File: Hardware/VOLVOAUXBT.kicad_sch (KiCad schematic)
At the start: 66 parts, among them J1 10118193-0001LF, J10 Conn_01x02_Pin, J11 Conn_01x02_Pin, J12 Conn_01x05_Pin, J13 Conn_01x05_Pin, J14 Conn_01x05_Pin, J15 Conn_01x02_Pin, J16 Conn_01x02_Pin, J17 Conn_01x01_Pin, J18 Conn_01x02_Pin, J19 Conn_01x01_Pin, J2 10118193-0001LF, J3 F52R-1A7H1-11018, J4 Conn_01x18_Pin, J5 Conn_01x18_Pin, J6 F52R-1A7H1-11018, J7 Conn_01x18_Pin, J8 U_FL-R-SMT_10_, J9 Conn_01x02_Pin, U1 SGM2212-3.3, U2 SGM2212-3.3, U3 TJA1027T_20_118, U4 ESP32-MINI-1, U5 TJA1027T_20_118, U6 SN74AHCT157PWR, U7 CP2102N-Axx-xQFN20

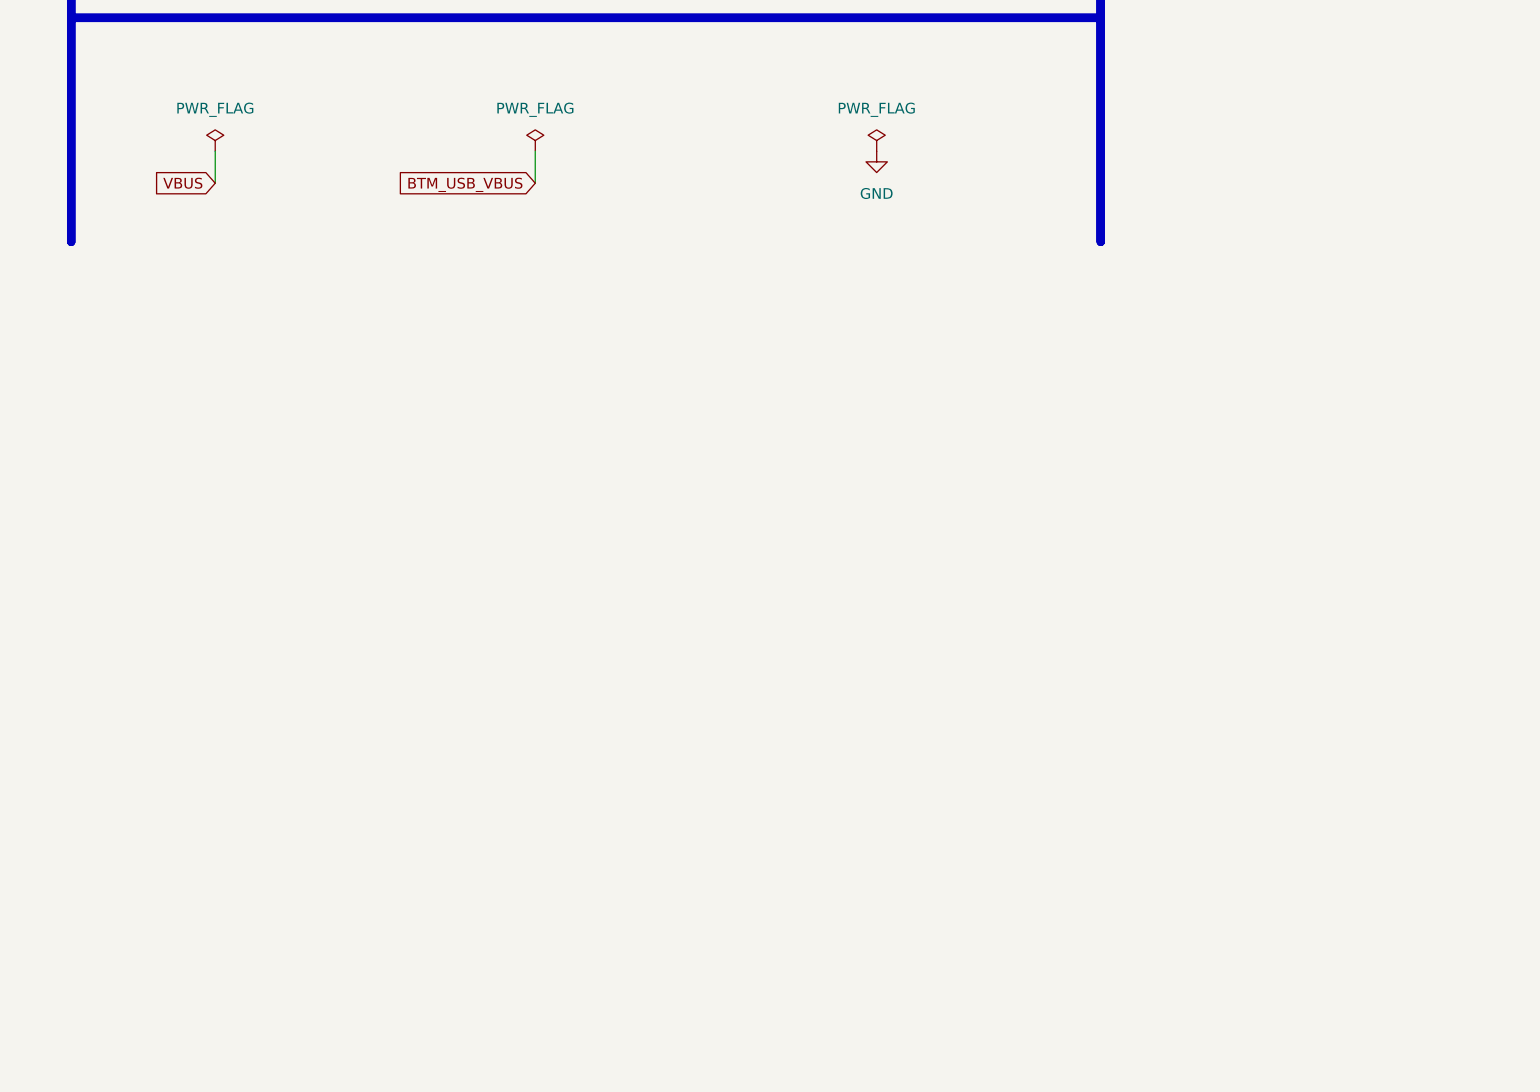
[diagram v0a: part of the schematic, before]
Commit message: Before swap to wroom
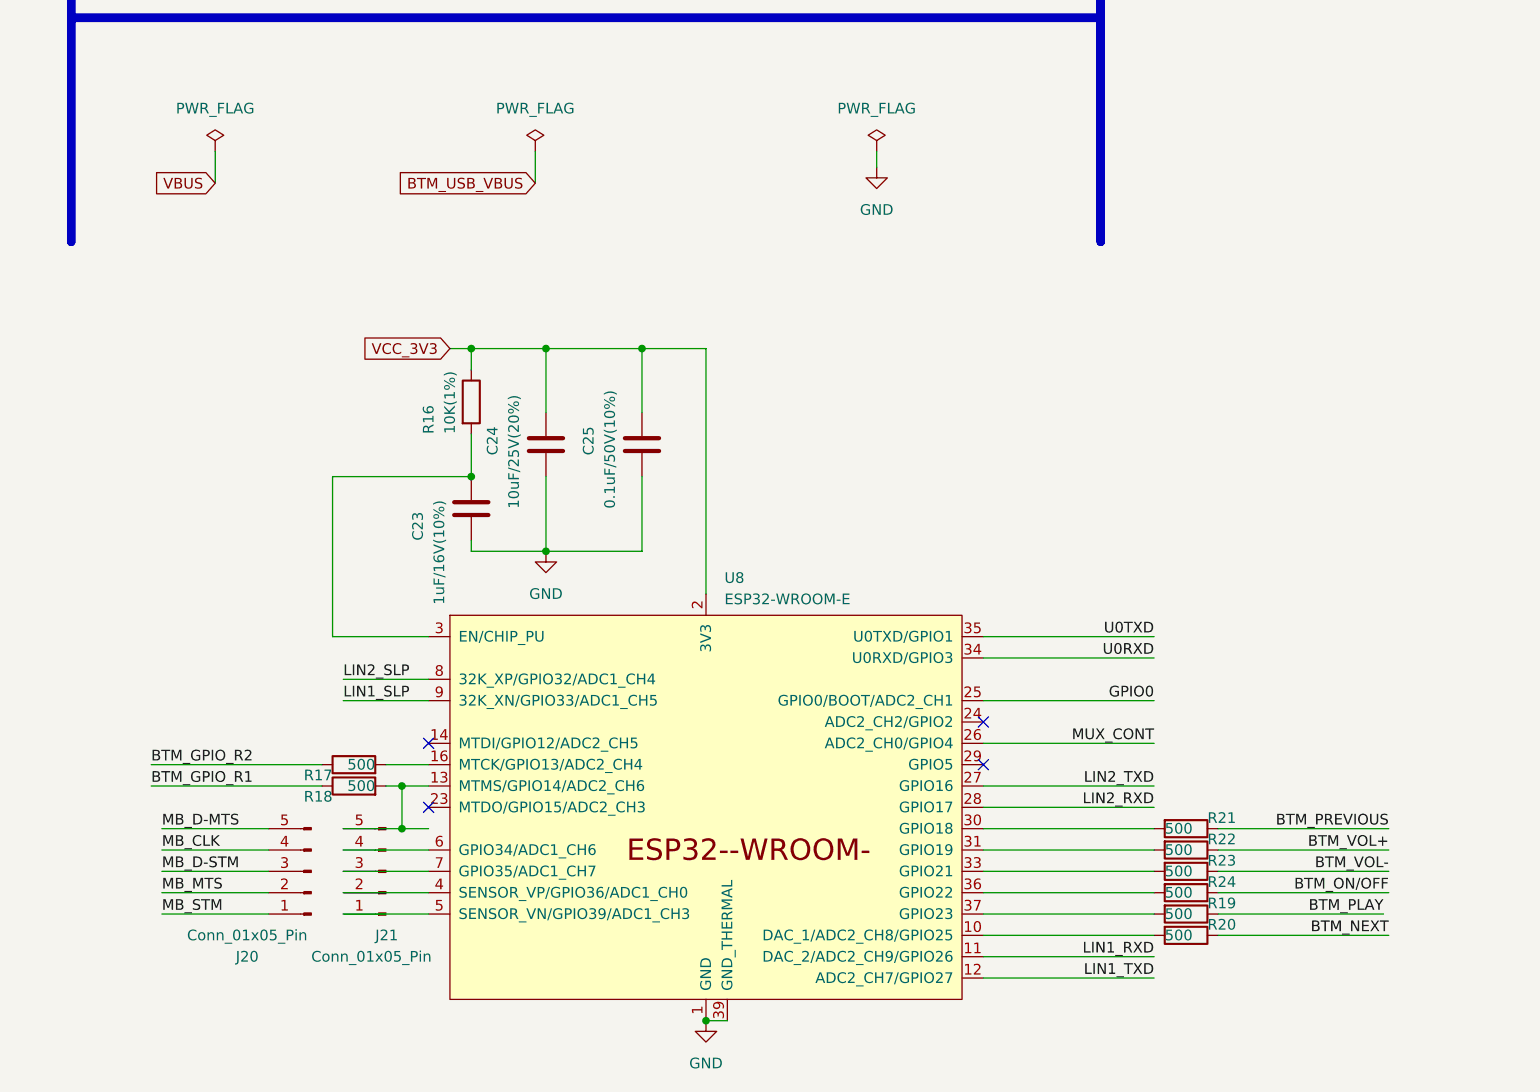
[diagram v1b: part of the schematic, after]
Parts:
- added C23: 1uF/16V(10%), Capacitor_SMD:C_1206_3216Metric, symbol Device:C
- added C24: 10uF/25V(20%), Capacitor_SMD:C_1206_3216Metric, symbol Device:C
- added C25: 0.1uF/50V(10%), Capacitor_SMD:C_1206_3216Metric, symbol Device:C
- added J20, J21: Conn_01x05_Pin, Connector_PinHeader_2.54mm:PinHeader_1x05_P2.54mm_Vertical, symbol Connector:Conn_01x05_Pin
- added R16: 10K(1%), Resistor_SMD:R_0603_1608Metric, symbol Device:R
- added R17, R18, R19, R20, R21, R22, R23, R24: 500, Resistor_SMD:R_0603_1608Metric, symbol Device:R
- added U8: ESP32-WROOM-E, PCM_Espressif:ESP32-WROOM-32E, symbol PCM_Espressif:ESP32-WROOM-E
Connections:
- net BTM_GPIO_R1: now also R18.1
- net BTM_GPIO_R2: now also R17.1
- net BTM_NEXT: now also R20.1
- net BTM_ON/OFF: now also R24.1
- net BTM_PLAY: now also R19.1
- net BTM_PREVIOUS: now also R21.1
- net BTM_VOL+: now also R22.1
- net BTM_VOL-: now also R23.1
- net GND: now also C23.2, C24.2, C25.2, U8.1 (GND), U8.15 (GND), U8.38 (GND), U8.39 (GND_THERMAL)
- net GPIO0: now also U8.25 (GPIO0/BOOT/ADC2_CH1)
- net LIN1_RXD: now also U8.11 (DAC_2/ADC2_CH9/GPIO26)
- net LIN1_SLP: now also U8.9 (32K_XN/GPIO33/ADC1_CH5)
- net LIN1_TXD: now also U8.12 (ADC2_CH7/GPIO27)
- net LIN2_RXD: now also U8.28 (GPIO17)
- net LIN2_SLP: now also U8.8 (32K_XP/GPIO32/ADC1_CH4)
- net LIN2_TXD: now also U8.27 (GPIO16)
- net MB_CLK: now also J20.4 (Pin_4)
- net MB_D-MTS: now also J20.5 (Pin_5)
- net MB_D-STM: now also J20.3 (Pin_3)
- net MB_MTS: now also J20.2 (Pin_2)
- net MB_STM: now also J20.1 (Pin_1)
- net MUX_CONT: now also U8.26 (ADC2_CH0/GPIO4)
- net U0RXD: now also U8.34 (U0RXD/GPIO3)
- net U0TXD: now also U8.35 (U0TXD/GPIO1)
- net VCC_3V3: now also C24.1, C25.1, R16.1, U8.2 (3V3)
- new net: R23.2, U8.33 (GPIO21)
- new net: R21.2, U8.30 (GPIO18)
- new net: R22.2, U8.31 (GPIO19)
- new net: R24.2, U8.36 (GPIO22)
- new net: J21.5 (Pin_5), R18.2, U8.13 (MTMS/GPIO14/ADC2_CH6)
- new net: J21.1 (Pin_1), U8.5 (SENSOR_VN/GPIO39/ADC1_CH3)
- new net: J21.2 (Pin_2), U8.4 (SENSOR_VP/GPIO36/ADC1_CH0)
- new net: J21.3 (Pin_3), U8.7 (GPIO35/ADC1_CH7)
- new net: J21.4 (Pin_4), U8.6 (GPIO34/ADC1_CH6)
- new net: R20.2, U8.10 (DAC_1/ADC2_CH8/GPIO25)
- new net: C23.1, R16.2, U8.3 (EN/CHIP_PU)
- new net: R19.2, U8.37 (GPIO23)
- new net: R17.2, U8.16 (MTCK/GPIO13/ADC2_CH4)
- no-connect marks 38 -> 42
